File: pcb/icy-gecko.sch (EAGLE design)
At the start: 64 parts, among them J1 USB-C, J2 8, J3 8, J4 8, J5 8, J6 4, J7 4, U1 EFM32GG12B8XX_QFN64, U2 ICE40LP384-SG32, U3 MIC23159, U6 SST26VF016B

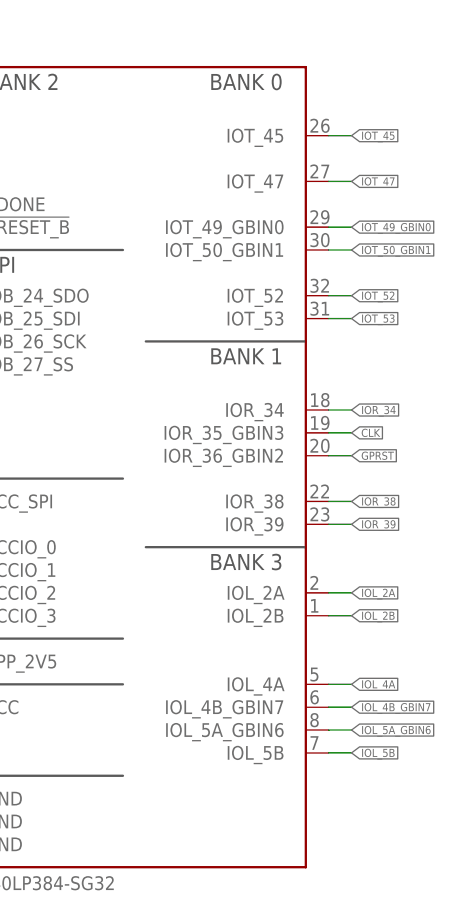
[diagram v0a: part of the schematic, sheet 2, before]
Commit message: sync
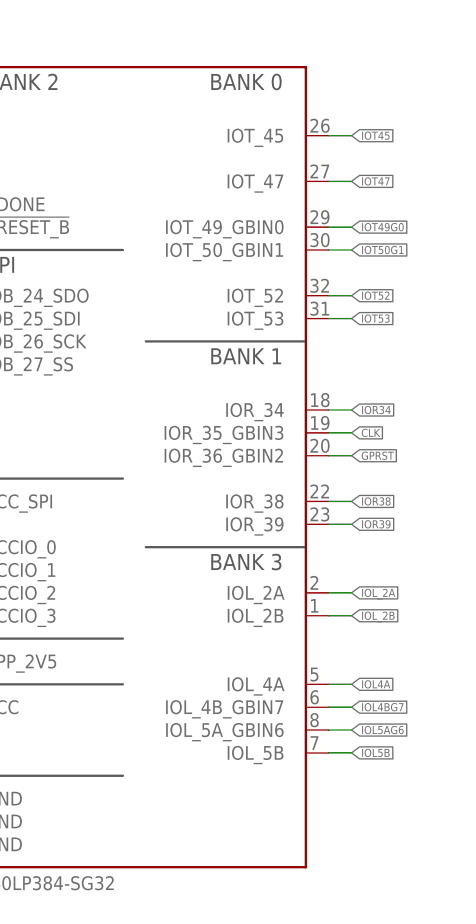
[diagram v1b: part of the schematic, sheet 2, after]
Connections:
- net IOL_4A renamed IOL4A
- net IOL_4B_GBIN7 renamed IOL4BG7
- net IOL_5A_GBIN6 renamed IOL5AG6
- net IOL_5B renamed IOL5B
- net IOR_34 renamed IOR34
- net IOR_38 renamed IOR38
- net IOR_39 renamed IOR39
- net IOT_45 renamed IOT45
- net IOT_47 renamed IOT47
- net IOT_49_GBIN0 renamed IOT49G0
- net IOT_50_GBIN1 renamed IOT50G1
- net IOT_52 renamed IOT52
- net IOT_53 renamed IOT53
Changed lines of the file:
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@@
 </segment>
 </net>
-<net name="IOT_45" class="0">
+<net name="IOT45" class="0">
 <segment>
 <wire x1="231.14" y1="154.94" x2="233.68" y2="154.94" width="0.1524" layer="91"/>
@@
 </segment>
 </net>
-<net name="IOT_47" class="0">
+<net name="IOT47" class="0">
 <segment>
 <wire x1="233.68" y1="149.86" x2="231.14" y2="149.86" width="0.1524" layer="91"/>
@@
 </segment>
 </net>
-<net name="IOT_49_GBIN0" class="0">
+<net name="IOT49G0" class="0">
 <segment>
 <wire x1="233.68" y1="144.78" x2="231.14" y2="144.78" width="0.1524" layer="91"/>
@@
 </segment>
 </net>
-<net name="IOT_50_GBIN1" class="0">
+<net name="IOT50G1" class="0">
 <segment>
 <wire x1="233.68" y1="142.24" x2="231.14" y2="142.24" width="0.1524" layer="91"/>
@@
 </segment>
 </net>
-<net name="IOT_52" class="0">
+<net name="IOT52" class="0">
 <segment>
 <wire x1="233.68" y1="137.16" x2="231.14" y2="137.16" width="0.1524" layer="91"/>
@@
 </segment>
 </net>
-<net name="IOT_53" class="0">
+<net name="IOT53" class="0">
 <segment>
 <wire x1="233.68" y1="134.62" x2="231.14" y2="134.62" width="0.1524" layer="91"/>
@@
 </segment>
 </net>
-<net name="IOR_38" class="0">
+<net name="IOR38" class="0">
 <segment>
 <wire x1="233.68" y1="114.3" x2="231.14" y2="114.3" width="0.1524" layer="91"/>
@@
 </segment>
 </net>
-<net name="IOR_39" class="0">
+<net name="IOR39" class="0">
 <segment>
 <wire x1="231.14" y1="111.76" x2="233.68" y2="111.76" width="0.1524" layer="91"/>
@@
 </segment>
 </net>
-<net name="IOL_4A" class="0">
+<net name="IOL4A" class="0">
 <segment>
 <wire x1="233.68" y1="93.98" x2="231.14" y2="93.98" width="0.1524" layer="91"/>
@@
 </segment>
 </net>
-<net name="IOL_4B_GBIN7" class="0">
+<net name="IOL4BG7" class="0">
 <segment>
 <wire x1="233.68" y1="91.44" x2="231.14" y2="91.44" width="0.1524" layer="91"/>
@@
 </segment>
 </net>
-<net name="IOL_5A_GBIN6" class="0">
+<net name="IOL5AG6" class="0">
 <segment>
 <wire x1="233.68" y1="88.9" x2="231.14" y2="88.9" width="0.1524" layer="91"/>
@@
 </segment>
 </net>
-<net name="IOL_5B" class="0">
+<net name="IOL5B" class="0">
 <segment>
 <wire x1="233.68" y1="86.36" x2="231.14" y2="86.36" width="0.1524" layer="91"/>
@@
 </segment>
 </net>
-<net name="IOR_34" class="0">
+<net name="IOR34" class="0">
 <segment>
 <pinref part="U2" gate="G$1" pin="IOR_34@18"/>
@@
 </segment>
 </net>
-<net name="IOL_4A" class="0">
+<net name="IOL4A" class="0">
 <segment>
 <wire x1="236.22" y1="101.6" x2="236.22" y2="99.06" width="0.1524" layer="91"/>
@@
 </segment>
 </net>
-<net name="IOL_4B_GBIN7" class="0">
+<net name="IOL4BG7" class="0">
 <segment>
 <wire x1="238.76" y1="101.6" x2="238.76" y2="99.06" width="0.1524" layer="91"/>
@@
 </segment>
 </net>
-<net name="IOL_5A_GBIN6" class="0">
+<net name="IOL5AG6" class="0">
 <segment>
 <wire x1="243.84" y1="101.6" x2="243.84" y2="99.06" width="0.1524" layer="91"/>
@@
 </segment>
 </net>
-<net name="IOL_5B" class="0">
+<net name="IOL5B" class="0">
 <segment>
 <wire x1="241.3" y1="101.6" x2="241.3" y2="99.06" width="0.1524" layer="91"/>
@@
 </segment>
 </net>
-<net name="IOT_52" class="0">
+<net name="IOT52" class="0">
 <segment>
 <wire x1="228.6" y1="101.6" x2="228.6" y2="99.06" width="0.1524" layer="91"/>
@@
 </segment>
 </net>
-<net name="IOT_45" class="0">
+<net name="IOT45" class="0">
 <segment>
 <wire x1="236.22" y1="160.02" x2="236.22" y2="157.48" width="0.1524" layer="91"/>
@@
 </segment>
 </net>
-<net name="IOT_47" class="0">
+<net name="IOT47" class="0">
 <segment>
 <wire x1="233.68" y1="157.48" x2="233.68" y2="160.02" width="0.1524" layer="91"/>
@@
 </segment>
 </net>
-<net name="IOT_49_GBIN0" class="0">
+<net name="IOT49G0" class="0">
 <segment>
 <wire x1="231.14" y1="157.48" x2="231.14" y2="160.02" width="0.1524" layer="91"/>
@@
 </segment>
 </net>
-<net name="IOT_50_GBIN1" class="0">
+<net name="IOT50G1" class="0">
 <segment>
 <wire x1="228.6" y1="157.48" x2="228.6" y2="160.02" width="0.1524" layer="91"/>
@@
 </segment>
 </net>
-<net name="IOT_53" class="0">
+<net name="IOT53" class="0">
 <segment>
 <wire x1="226.06" y1="157.48" x2="226.06" y2="160.02" width="0.1524" layer="91"/>
@@
 </segment>
 </net>
-<net name="IOR_38" class="0">
+<net name="IOR38" class="0">
 <segment>
 <wire x1="241.3" y1="157.48" x2="241.3" y2="160.02" width="0.1524" layer="91"/>
@@
 </segment>
 </net>
-<net name="IOR_34" class="0">
+<net name="IOR34" class="0">
 <segment>
 <wire x1="243.84" y1="160.02" x2="243.84" y2="157.48" width="0.1524" layer="91"/>
@@
 </segment>
 </net>
-<net name="IOR_39" class="0">
+<net name="IOR39" class="0">
 <segment>
 <wire x1="238.76" y1="160.02" x2="238.76" y2="157.48" width="0.1524" layer="91"/>
